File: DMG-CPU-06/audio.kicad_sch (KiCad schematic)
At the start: 12 parts, among them J3 Conn_01x04, U4 IR3R40N

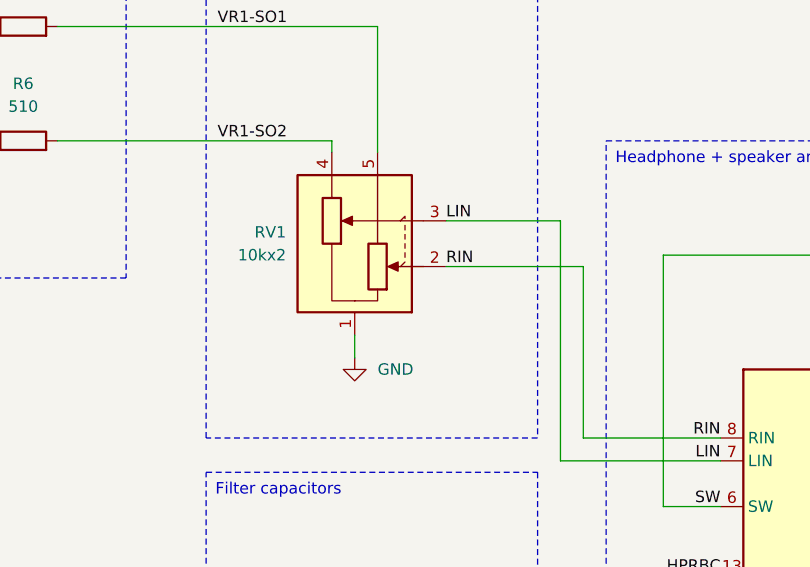
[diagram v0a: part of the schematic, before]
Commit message: Tidy up potentiometer symbols, add contrast pot symbols
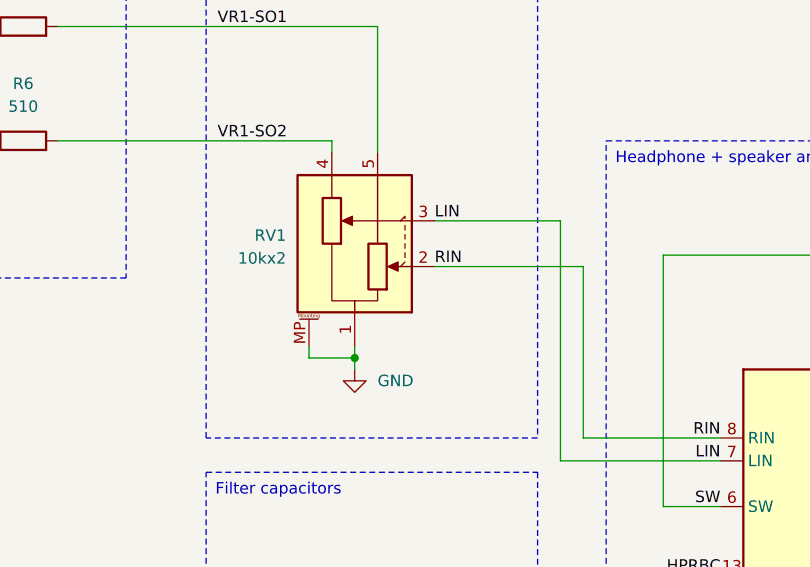
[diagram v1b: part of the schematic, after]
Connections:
- net GND: now also RV1.MP (MountPin)
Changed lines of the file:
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@@
   (junction (at 133.35 137.16) (diameter 0) (color 0 0 0 0)
+  )
+  (junction (at 80.01 95.25) (diameter 0) (color 0 0 0 0)
   )
   (no_connect (at 120.65 124.46))
@@
     (stroke (width 0) (type default))
   )
+  (wire (pts (xy 80.01 93.98) (xy 80.01 95.25))
+    (stroke (width 0) (type default))
+  )
   (wire (pts (xy 85.09 134.62) (xy 85.09 133.35))
     (stroke (width 0) (type default))
@@
     (stroke (width 0) (type default))
   )
-  (wire (pts (xy 90.17 85.09) (xy 105.41 85.09))
+  (wire (pts (xy 88.9 85.09) (xy 105.41 85.09))
     (stroke (width 0) (type default))
   )
@@
     (stroke (width 0) (type default))
   )
-  (wire (pts (xy 80.01 92.71) (xy 80.01 95.25))
-    (stroke (width 0) (type default))
-  )
   (wire (pts (xy 135.89 134.62) (xy 135.89 137.16))
     (stroke (width 0) (type default))
@@
     (stroke (width 0) (type default))
   )
+  (wire (pts (xy 80.01 95.25) (xy 80.01 96.52))
+    (stroke (width 0) (type default))
+  )
   (wire (pts (xy 114.3 83.82) (xy 196.85 83.82))
     (stroke (width 0) (type default))
@@
     (stroke (width 0) (type default))
   )
-  (wire (pts (xy 90.17 80.01) (xy 102.87 80.01))
+  (wire (pts (xy 88.9 80.01) (xy 102.87 80.01))
     (stroke (width 0) (type default))
   )
@@
   )
   (wire (pts (xy 146.05 137.16) (xy 135.89 137.16))
+    (stroke (width 0) (type default))
+  )
+  (wire (pts (xy 74.93 93.98) (xy 74.93 95.25))
+    (stroke (width 0) (type default))
+  )
+  (wire (pts (xy 74.93 95.25) (xy 80.01 95.25))
     (stroke (width 0) (type default))
   )
@@
     (effects (font (size 1.27 1.27)) (justify left bottom))
   )
-  (label "RIN" (at 90.17 85.09 0) (fields_autoplaced)
+  (label "RIN" (at 88.9 85.09 0) (fields_autoplaced)
     (effects (font (size 1.27 1.27)) (justify left bottom))
   )
-  (label "LIN" (at 90.17 80.01 0) (fields_autoplaced)
+  (label "LIN" (at 88.9 80.01 0) (fields_autoplaced)
     (effects (font (size 1.27 1.27)) (justify left bottom))
   )
@@
     )
   )
-  (symbol (lib_id "power:GND") (at 80.01 95.25 0) (unit 1)
-    (in_bom yes) (on_board yes) (dnp no) (fields_autoplaced)
-    (property "Reference" "#PWR0134" (at 80.01 101.6 0)
-      (effects (font (size 1.27 1.27)) hide)
-    )
-    (property "Value" "GND" (at 82.55 96.52 0)
-      (effects (font (size 1.27 1.27)) (justify left))
-    )
-    (property "Footprint" "" (at 80.01 95.25 0)
-      (effects (font (size 1.27 1.27)) hide)
-    )
-    (property "Datasheet" "" (at 80.01 95.25 0)
+  (symbol (lib_id "power:GND") (at 80.01 96.52 0) (unit 1)
+    (in_bom yes) (on_board yes) (dnp no) (fields_autoplaced)
+    (property "Reference" "#PWR0134" (at 80.01 102.87 0)
+      (effects (font (size 1.27 1.27)) hide)
+    )
+    (property "Value" "GND" (at 82.55 97.79 0)
+      (effects (font (size 1.27 1.27)) (justify left))
+    )
+    (property "Footprint" "" (at 80.01 96.52 0)
+      (effects (font (size 1.27 1.27)) hide)
+    )
+    (property "Datasheet" "" (at 80.01 96.52 0)
       (effects (font (size 1.27 1.27)) hide)
     )
@@
     )
   )
-  (symbol (lib_id "Gekkio_Device_Specialized:R_Potentiometer_GameBoy_Volume_DMG") (at 80.01 82.55 270) (mirror x) (unit 1)
-    (in_bom yes) (on_board yes) (dnp no) (fields_autoplaced)
-    (property "Reference" "RV1" (at 72.39 81.28 90)
-      (effects (font (size 1.27 1.27)) (justify right))
-    )
-    (property "Value" "10kx2" (at 72.39 83.82 90)
-      (effects (font (size 1.27 1.27)) (justify right))
-    )
-    (property "Footprint" "" (at 78.105 78.74 0)
-      (effects (font (size 1.27 1.27)) hide)
-    )
-    (property "Datasheet" "" (at 78.105 78.74 0)
+  (symbol (lib_id "Gekkio_Device_Specialized:R_Potentiometer_GameBoy_Volume_DMG") (at 80.01 82.55 0) (mirror y) (unit 1)
+    (in_bom yes) (on_board yes) (dnp no) (fields_autoplaced)
+    (property "Reference" "RV1" (at 72.39 81.6356 0)
+      (effects (font (size 1.27 1.27)) (justify left))
+    )
+    (property "Value" "10kx2" (at 72.39 84.1756 0)
+      (effects (font (size 1.27 1.27)) (justify left))
+    )
+    (property "Footprint" "" (at 76.2 84.455 0)
+      (effects (font (size 1.27 1.27)) hide)
+    )
+    (property "Datasheet" "" (at 76.2 84.455 0)
       (effects (font (size 1.27 1.27)) hide)
     )
@@
     (pin "4")
     (pin "5")
-    (instances
-      (project "DMG-CPU-06"
+    (pin "MP")
+    (instances
+      (project "DMG-CPU-06"
